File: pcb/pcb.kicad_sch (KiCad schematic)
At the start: 21 parts, among them J1 USB_C_Receptacle_USB2.0_14P, U1 RP2040, U2 NCP1117-3.3_SOT223

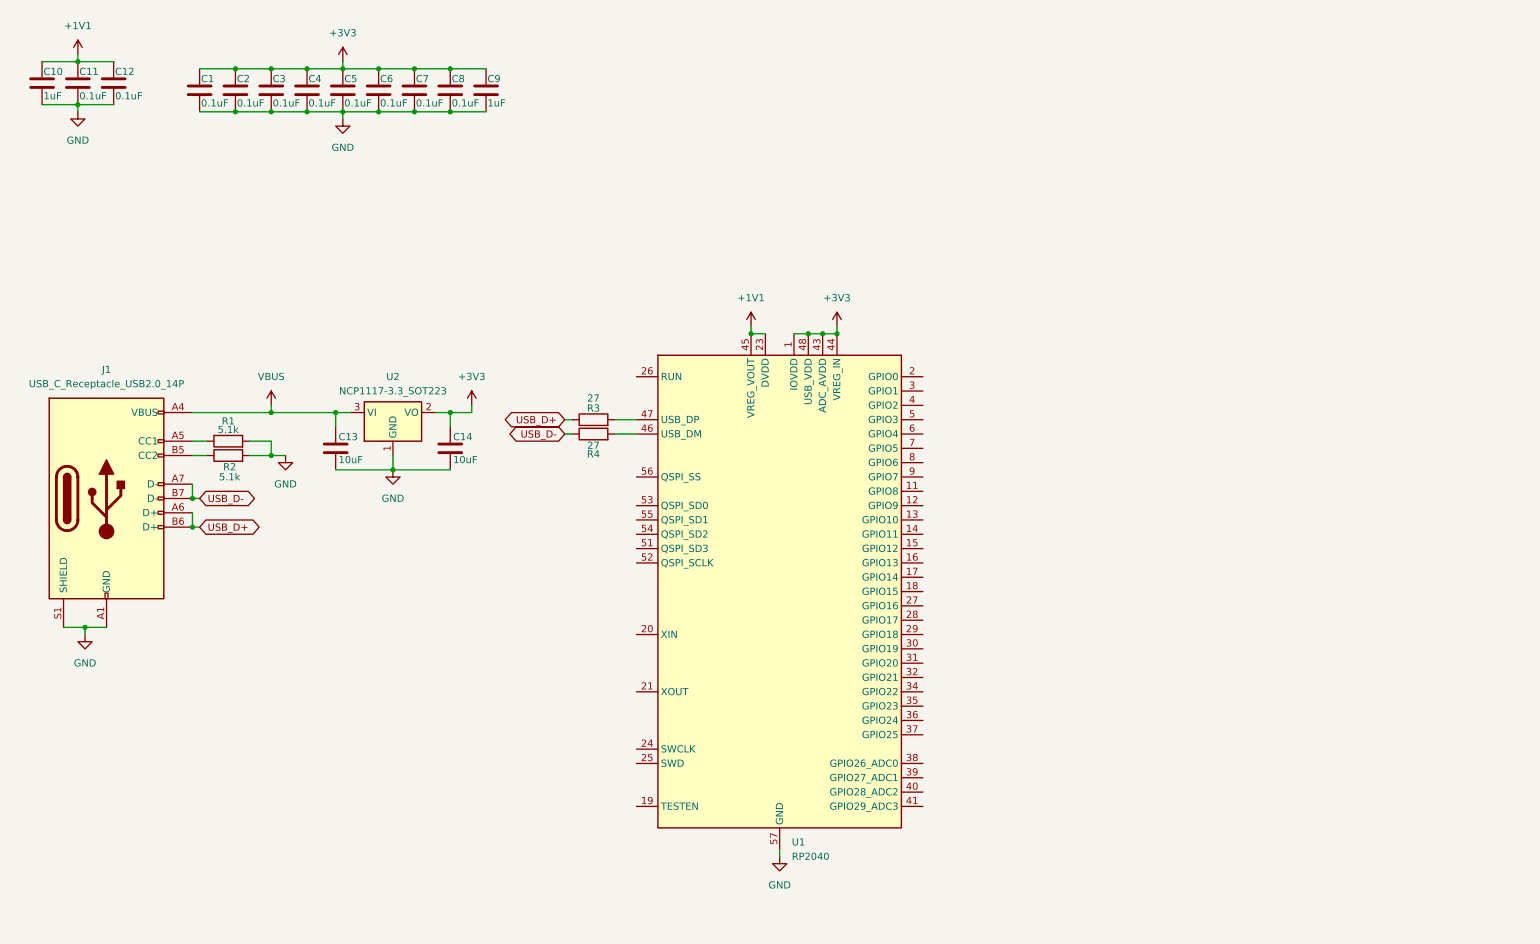
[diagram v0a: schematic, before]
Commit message: logging off for the night - completed the schematic
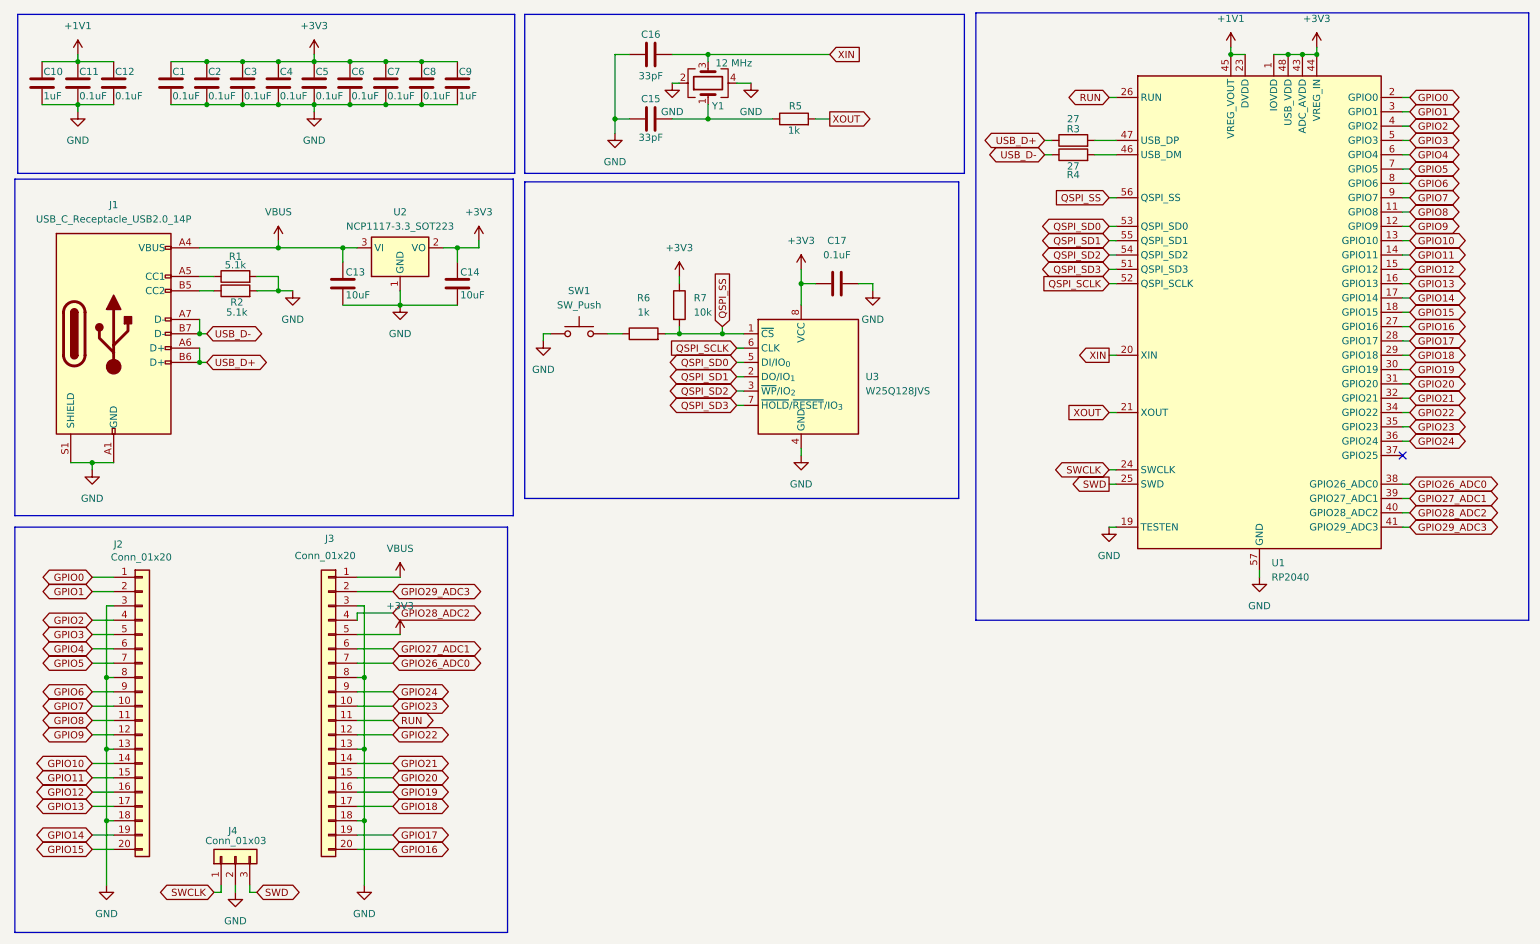
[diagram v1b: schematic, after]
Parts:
- added C15, C16: 33pF, Capacitor_SMD:C_0402_1005Metric, symbol Device:C
- added C17: 0.1uF, Capacitor_SMD:C_0402_1005Metric, symbol Device:C
- added J2, J3: Conn_01x20, Connector_PinHeader_2.54mm:PinHeader_1x20_P2.54mm_Vertical, symbol Connector_Generic:Conn_01x20
- added J4: Conn_01x03, Connector_PinHeader_2.54mm:PinHeader_1x03_P2.54mm_Vertical, symbol Connector_Generic:Conn_01x03
- added R5, R6: 1k, Resistor_SMD:R_0402_1005Metric, symbol Device:R
- added R7: 10k, Resistor_SMD:R_0402_1005Metric, symbol Device:R
- added SW1: SW_Push, Button_Switch_SMD:SW_Push_SPST_NO_Alps_SKRK, symbol Switch:SW_Push
- added U3: W25Q128JVS, Package_SO:SOIC-8_5.3x5.3mm_P1.27mm, symbol Memory_Flash:W25Q128JVS
- added Y1: 12 MHz, Crystal:Crystal_SMD_3225-4Pin_3.2x2.5mm, symbol Device:Crystal_GND24
- C1, C10, C11, C12, C13, C14, C2, C3, C4, C5, C6, C7, C8, C9: footprint (none) -> Capacitor_SMD:C_0402_1005Metric
- J1: footprint (none) -> Connector_USB:USB_C_Receptacle_HRO_TYPE-C-31-M-12
- R1, R2, R3, R4: footprint (none) -> Resistor_SMD:R_0402_1005Metric
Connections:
- net +3V3: now also C17.1, J3.5 (Pin_5), R7.1, U3.8 (VCC)
- net GND: now also U1.19 (TESTEN), C15.1, C16.1, C17.2, J2.13 (Pin_13), J2.18 (Pin_18), J2.3 (Pin_3), J2.8 (Pin_8), J3.13 (Pin_13), J3.18 (Pin_18), J3.3 (Pin_3), J3.8 (Pin_8), J4.2 (Pin_2), SW1.1, U3.4 (GND), Y1.2, Y1.4
- net VBUS: now also J3.1 (Pin_1)
- net GPIO8: now reaches U1.11 (GPIO8)
- net GPIO8: now also J2.11 (Pin_11)
- net GPIO9: now reaches U1.12 (GPIO9)
- net GPIO9: now also J2.12 (Pin_12)
- net GPIO10: now reaches U1.13 (GPIO10)
- net GPIO10: now also J2.14 (Pin_14)
- net GPIO11: now reaches U1.14 (GPIO11)
- net GPIO11: now also J2.15 (Pin_15)
- net GPIO12: now reaches U1.15 (GPIO12)
- net GPIO12: now also J2.16 (Pin_16)
- net GPIO13: now reaches U1.16 (GPIO13)
- net GPIO13: now also J2.17 (Pin_17)
- net GPIO14: now reaches U1.17 (GPIO14)
- net GPIO14: now also J2.19 (Pin_19)
- net GPIO15: now reaches U1.18 (GPIO15)
- net GPIO15: now also J2.20 (Pin_20)
- net GPIO0: now reaches U1.2 (GPIO0)
- net GPIO0: now also J2.1 (Pin_1)
- net XIN: now reaches U1.20 (XIN)
- net XIN: now also C16.2, Y1.3
- net XOUT: now reaches U1.21 (XOUT)
- net XOUT: now also R5.2
- net SWCLK: now reaches U1.24 (SWCLK)
- net SWCLK: now also J4.1 (Pin_1)
- net SWD: now reaches U1.25 (SWD)
- net SWD: now also J4.3 (Pin_3)
- net RUN: now reaches U1.26 (RUN)
- net RUN: now also J3.11 (Pin_11)
- net GPIO16: now reaches U1.27 (GPIO16)
- net GPIO16: now also J3.20 (Pin_20)
- net GPIO17: now reaches U1.28 (GPIO17)
- net GPIO17: now also J3.19 (Pin_19)
- net GPIO18: now reaches U1.29 (GPIO18)
- net GPIO18: now also J3.17 (Pin_17)
- net GPIO1: now reaches U1.3 (GPIO1)
- net GPIO1: now also J2.2 (Pin_2)
- net GPIO19: now reaches U1.30 (GPIO19)
- net GPIO19: now also J3.16 (Pin_16)
- net GPIO20: now reaches U1.31 (GPIO20)
- net GPIO20: now also J3.15 (Pin_15)
- net GPIO21: now reaches U1.32 (GPIO21)
- net GPIO21: now also J3.14 (Pin_14)
- net GPIO22: now reaches U1.34 (GPIO22)
- net GPIO22: now also J3.12 (Pin_12)
- net GPIO23: now reaches U1.35 (GPIO23)
- net GPIO23: now also J3.10 (Pin_10)
- net GPIO24: now reaches U1.36 (GPIO24)
- net GPIO24: now also J3.9 (Pin_9)
- net GPIO26_ADC0: now reaches U1.38 (GPIO26_ADC0)
- net GPIO26_ADC0: now also J3.7 (Pin_7)
- net GPIO27_ADC1: now reaches U1.39 (GPIO27_ADC1)
- net GPIO27_ADC1: now also J3.6 (Pin_6)
- net GPIO2: now reaches U1.4 (GPIO2)
- net GPIO2: now also J2.4 (Pin_4)
- net GPIO28_ADC2: now reaches U1.40 (GPIO28_ADC2)
- net GPIO28_ADC2: now also J3.4 (Pin_4)
- net GPIO29_ADC3: now reaches U1.41 (GPIO29_ADC3)
- net GPIO29_ADC3: now also J3.2 (Pin_2)
- net GPIO3: now reaches U1.5 (GPIO3)
- net GPIO3: now also J2.5 (Pin_5)
- net QSPI_SD3: now reaches U1.51 (QSPI_SD3)
- net QSPI_SD3: now also U3.7 (~{HOLD}/~{RESET}/IO_{3})
- net QSPI_SCLK: now reaches U1.52 (QSPI_SCLK)
- net QSPI_SCLK: now also U3.6 (CLK)
- net QSPI_SD0: now reaches U1.53 (QSPI_SD0)
- net QSPI_SD0: now also U3.5 (DI/IO_{0})
- net QSPI_SD2: now reaches U1.54 (QSPI_SD2)
- net QSPI_SD2: now also U3.3 (~{WP}/IO_{2})
- net QSPI_SD1: now reaches U1.55 (QSPI_SD1)
- net QSPI_SD1: now also U3.2 (DO/IO_{1})
- net QSPI_SS: now reaches U1.56 (QSPI_SS)
- net QSPI_SS: now also R6.2, R7.2, U3.1 (~{CS})
- net GPIO4: now reaches U1.6 (GPIO4)
- net GPIO4: now also J2.6 (Pin_6)
- net GPIO5: now reaches U1.7 (GPIO5)
- net GPIO5: now also J2.7 (Pin_7)
- net GPIO6: now reaches U1.8 (GPIO6)
- net GPIO6: now also J2.9 (Pin_9)
- net GPIO7: now reaches U1.9 (GPIO7)
- net GPIO7: now also J2.10 (Pin_10)
- new net: R6.1, SW1.2
- new net: C15.2, R5.1, Y1.1
- no-connect marks 0 -> 1
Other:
- moved on the sheet: C1, C13, C14, C2, C3, C4, C5, C6, C7, C8, C9, J1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
